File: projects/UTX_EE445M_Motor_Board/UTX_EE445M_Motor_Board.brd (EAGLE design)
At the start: 38.9 x 46 mm, 12 parts

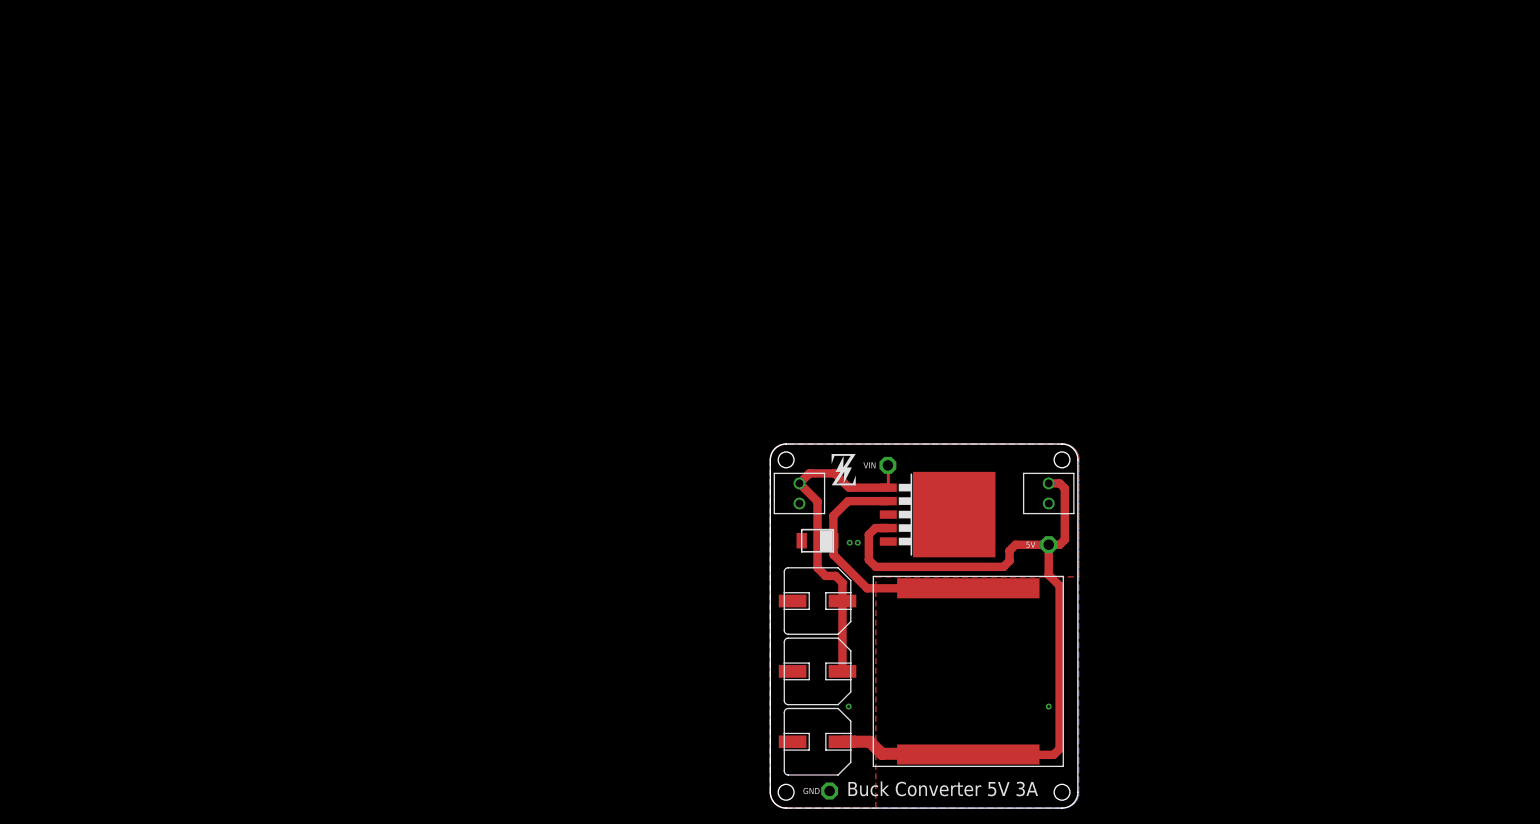
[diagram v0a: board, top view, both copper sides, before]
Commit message: add EE445M motor board
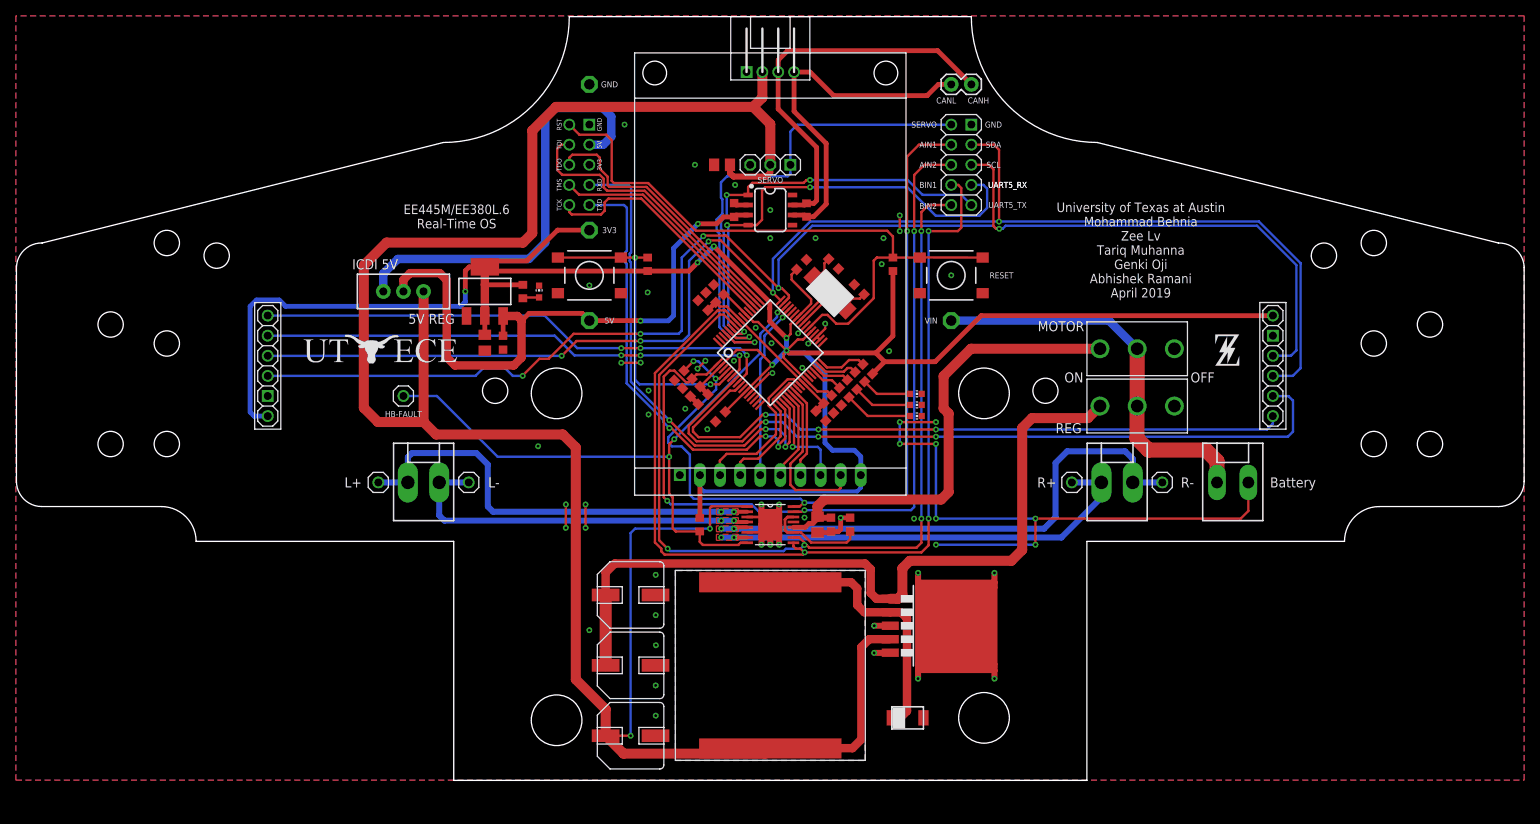
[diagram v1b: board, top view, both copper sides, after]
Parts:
- removed U$22: POWER_CONNECTOR, Z:_TERMINAL_BLOCK_2.54_1X2
- added 3V3: TPPAD1-13, testpad:P1-13
- added BUTTON, RESET: _SWITCH_DTSM-6, Z:_SWITCH_DTSM-6
- added C10, C17, C21, C6, C9: 0.1uF, UT_ECE:C0603K
- added C11, C7: 1uF, UT_ECE:C0603K
- added C12: (no value), UT_ECE:C0805K
- added C13: (no value), UT_ECE:C0603K
- added C14, C15, C16: 330uF, 35V, Z:_CAPACITOR_CHEMI-CON_A_HA0_SMD
- added C18, C19: 2.2uF, UT_ECE:C0603K
- added C20: 10uF, EE445L:C0805K
- added C22: 47uF, UT_ECE:C0805K
- added C3, C5, C8: 0.01uF, UT_ECE:C0603K
- added DIS1: ST7735, UT_ECE:ST7735
- added HB-FAULT, L+, L-, R+, R-: (no value), EE445L:1X01
- added IC2: (no value), Z:_PACKAGE_TO263-5
- added JP1: (no value), UT_ECE:1X02
- added LED1, LED2, LED3, PWR_LED: (no value), led:CHIP-LED0603
- added Q1: NX5032GA, UT_ECE:NX5032GA
- added R1, R2, R4: 470, UT_ECE:R0603
- added R10, R11, R7, R8, R9: 10k, UT_ECE:R0603
- added R3: 470, rcl:R0603
- added R5: 1M, UT_ECE:R0603
- added R6: 120, UT_ECE:R0603
- added S1: (no value), SparkFun-Switches:SWITCH_SPDT_PTH_11.6X4.0MM
- added SERVO: (no value), EE445L:1X03
- added U$10: UTX_EE445M_BOARD_CONNECTOR, Z:_HEADER_2_4X1_ANGLED
- added U$11: LOGIC_ANALYZER_10PIN, Z:LOGIC_ANALYZER_10PIN
- added U$3: LIDAR_VL53L0X_ATK_VERT, Z:LIDAR_VL53L0X_ATK_VERT
- added U$4, U$5: _SWITCH_SPDT_4.7, Z:_SWITCH_SPDT_4.7
- added U$6: (no value), Z:__LOGO_UT_ECE
- added U$7: (no value), Z:__LOGO_Z
- added U$9: _VOLTAGE_REGULATOR_AMS1117, Z:_PACKAGE_SOT223
- added U1: DRV8848, UT_ECE:SOP65P640X120-17N
- added U4: MCP2551PSOIC, UT_ECE:SO08
- added X1, X2: (no value), EE445L:KK-156-2
- added X3: (no value), UT_ECE:KK-156-2
- C1, C2: value 330uF, 35V -> 10pF; device Z:_CAPACITOR_CHEMI-CON_A_HA0_SMD -> UT_ECE:C0603K
- C4: value 330uF, 35V -> 0.1uF; device Z:_CAPACITOR_CHEMI-CON_A_HA0_SMD -> UT_ECE:C0603K
- IC1: value (none) -> TM4C123GH6PM; device Z:_PACKAGE_TO263-5 -> UT_ECE:SQFP-S-10X10-64
- U$1: value POWER_CONNECTOR -> JTAG_SERIAL; device Z:_TERMINAL_BLOCK_2.54_1X2 -> Z:JTAG_SERIAL_PTH
- U$2: value (none) -> LIDAR_VL53L0X_ATK_VERT; device Z:__LOGO_Z -> Z:LIDAR_VL53L0X_ATK_VERT
- moved GND 94.3 mm to (-22.9, 91.4)
- moved U$1 72.4 mm to (-24.1, 81.3)
- moved 5V 64.6 mm to (-22.9, 61.6)
- moved C4 58.5 mm to (-6.52, 65.5), turned to 135 degrees
- moved U$2 57.8 mm to (63.5, 55.9), turned to 270 degrees
- moved C2 51.5 mm to (7.99, 68.8), turned to 315 degrees
- moved C1 39.7 mm to (11.2, 65.5), turned to 135 degrees
- moved IC1 29.1 mm to (0.00, 57.5), turned to 315 degrees
- moved U$24 25.1 mm to (17.3, 11.4), turned to 180 degrees
- moved U$23 25.0 mm to (0.00, 18.0)
- moved VIN 20.0 mm to (22.9, 61.6)
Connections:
- new net 3V3: 3V3.TP, C12.1, C3.1, C4.1, C5.1, C6.1, C7.1, C8.1, DIS1.10, DIS1.2, IC1.11, IC1.2, IC1.26, IC1.37, IC1.42, IC1.54, R3.2, R5.1, R7.1, R8.1, R9.2, U$2.VCC, U$3.VCC, U$9.2, U$9.4
- new net 5V_REG: C14.+, C22.1, IC2.4, S1.1, SERVO.2, U$10.3, U$23.2, U1.1
- new net AIN1: IC1.4, R10.2, U$11.2, U1.16
- new net AIN2: IC1.1, R11.2, U$11.3, U1.15
- new net BIN1: IC1.57, U$11.4, U1.9
- new net BIN2: IC1.58, U$11.5, U1.10
- new net CANH: JP1.2, R6.2, U$10.2, U4.7
- new net CANL: JP1.1, R6.1, U$10.1, U4.6
- new net I2C0_SCL: IC1.47, U$11.8, U$2.SCL, U$3.SCL
- new net I2C0_SDA: IC1.48, U$11.9, U$2.SDA, U$3.SDA
- new net ICDI_5V: S1.3, U$1.5V
- new net L+: L+.1, U1.2, X1.1
- new net L-: L-.1, U1.4, X1.2
- new net N$1: U$1.3V3
- new net N$12: U$5.P$3
- new net N$19: IC1.32, R5.2
- new net N$4: LED1.A, R1.1
- new net N$6: PWR_LED.A, R3.1
- new net N$7: LED2.A, R2.1
- new net N$8: LED3.A, R4.1
- new net N$9: U$4.P$3
- new net NFAULT: HB-FAULT.1, IC1.46, R9.1, U1.8
- new net OSC0: C1.1, IC1.40, Q1.1
- new net OSC1: C2.1, IC1.41, Q1.2
- new net PF1: IC1.29, R1.2
- new net PF2: IC1.30, R2.2
- new net PF3: IC1.31, R4.2
- new net PF4: BUTTON.1, BUTTON.2, IC1.5, R8.2
- new net R+: R+.1, U1.7, X2.1
- new net R-: R-.1, U1.5, X2.2
- new net RST: IC1.38, R7.2, RESET.1, RESET.2, U$1.RST
- new net RXD: IC1.18, U$1.RXD
- new net SD_CS: DIS1.5, IC1.45
- new net SERVO_PWM: IC1.61, SERVO.1, U$11.1
- new net SSI0_MISO: DIS1.9, IC1.21
- new net SSI0_MOSI: DIS1.7, IC1.22
- new net SSI0_SCK: DIS1.8, IC1.19
- new net TCK: IC1.52, U$1.TCK
- new net TDI: IC1.50, U$1.TDI
- new net TDO: IC1.49, U$1.TDO
- new net TFT_CS: DIS1.6, IC1.20
- new net TFT_D/C: DIS1.4, IC1.23
- new net TFT_RESET: DIS1.3, IC1.24
- new net TMS: IC1.51, U$1.TMS
- new net TXD: IC1.17, U$1.TXD
- new net UART5_RX: IC1.59, U$11.7, U4.4
- new net UART5_TX: IC1.60, U$11.6, U4.1
- new net VDDC: C10.1, C11.1, C18.1, C9.1, IC1.25, IC1.56
- new net VINT: C19.1, U1.11, U1.14
- new net VIN_REG: C15.+, C16.+, IC2.1, U$5.P$1
- new net VX_INT1: IC1.7, U$2.INT
- new net VX_INT2: IC1.6, U$3.INT
- new net V_HB: C20.1, C21.1, U$4.P$1, U1.12
- new net XSHUT1: IC1.9, U$2.XSH
- new net XSHUT2: IC1.8, U$3.XSH
- net 5V: now also C13.1, C17.1, S1.2, U$9.3, U4.3; no longer C4.+, IC1.4, U$1.2, U$23.2
- net GND: now also BUTTON.3, BUTTON.4, C1.2, C10.2, C11.2, C12.2, C13.2, C14.-, C15.-, C16.-, C17.2, C18.2, C19.2, C2.2, C20.2, C21.2, C22.2, C3.2, C4.2, C5.2, C6.2, C7.2, C8.2, C9.2, DIS1.1, IC1.12, IC1.27, IC1.34, IC1.35, IC1.39, IC1.55, IC2.3, IC2.5, IC2.6, LED1.C, LED2.C, LED3.C, PWR_LED.C, R10.1, R11.1, RESET.3, RESET.4, SERVO.3, U$1.GND, U$10.4, U$11.10, U$2.GND, U$3.GND, U$9.1, U1.13, U1.17, U1.3, U1.6, U4.2, U4.8, X3.2; no longer C1.-, C2.-, C4.-, IC1.5, IC1.6, U$1.1, U$22.2
- net N$11: now also IC2.2; no longer IC1.2
- net VIN: now also U$4.P$2, U$5.P$2, X3.1; no longer C1.+, C2.+, IC1.1, U$22.1
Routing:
- net 3V3: track 0.00 -> 315.5 mm, vias 0 -> 6
- net 5V_REG: track 0.00 -> 283.2 mm, vias 0 -> 2
- net GND: track 0.00 -> 193.8 mm, vias 4 -> 63
- net I2C0_SDA: track 0.00 -> 184.6 mm, vias 0 -> 5
- net I2C0_SCL: track 0.00 -> 182.1 mm, vias 0 -> 5
- net BIN1: track 0.00 -> 124.3 mm, vias 0 -> 3
- net BIN2: track 0.00 -> 116.5 mm, vias 0 -> 4
- net AIN1: track 0.00 -> 105.6 mm, vias 0 -> 4
- net AIN2: track 0.00 -> 105.3 mm, vias 0 -> 3
- net VIN_REG: track 0.00 -> 99.3 mm
- net VX_INT1: track 0.00 -> 94.7 mm, vias 0 -> 3
- net XSHUT1: track 0.00 -> 85.5 mm, vias 0 -> 3
- net NFAULT: track 0.00 -> 82.5 mm, vias 0 -> 3
- net RST: track 0.00 -> 82.2 mm
- net R-: track 0.00 -> 68.9 mm, vias 0 -> 2
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- added copper zone on layer 1, net L+
- added copper zone on layer 1, net L-
- added copper zone on layer 1, net R+
- added copper zone on layer 1, net R-
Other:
- board size 38.9 x 46 mm -> 190.5 x 96.5 mm
- board text added: "5V REG"
- board text added: "AIN1"
- board text added: "AIN2"
- board text added: "BIN1"
- board text added: "BIN2"
- board text added: "Battery"
- board text added: "CANH"
- board text added: "CANL"
- board text added: "EE445M/EE380L.6 Real-Time OS"
- board text added: "GND"
- board text added: "ICDI 5V"
- board text added: "MOTOR"
- board text added: "OFF"
- board text added: "ON"
- board text added: "REG"
- board text added: "SCL"
- board text added: "SDA"
- board text added: "SERVO"
- board text added: "UART5_RX"
- board text added: "UART5_TX"
- board text added: "University of Texas at Austin Mohammad Behnia Zee Lv Tariq Muhanna Genki Oji Abhishek Ramani April 2019"
- board text removed: "Buck Converter 5V 3A"
- board text removed: "Mar 2019 Zee Lv"
